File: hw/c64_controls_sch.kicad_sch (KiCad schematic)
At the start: 22 parts, among them J300 DE9_Receptacle, J301 DE9_Receptacle, U300 74AHCT1G125, U301 74AHCT1G125, U302 74AHCT1G125, U303 74AHCT1G125, U304 74AHCT1G125, U305 74AHCT1G125, U306 74AHCT1G125, U307 74AHCT1G125, U308 74AHCT1G125, U309 74AHCT1G125

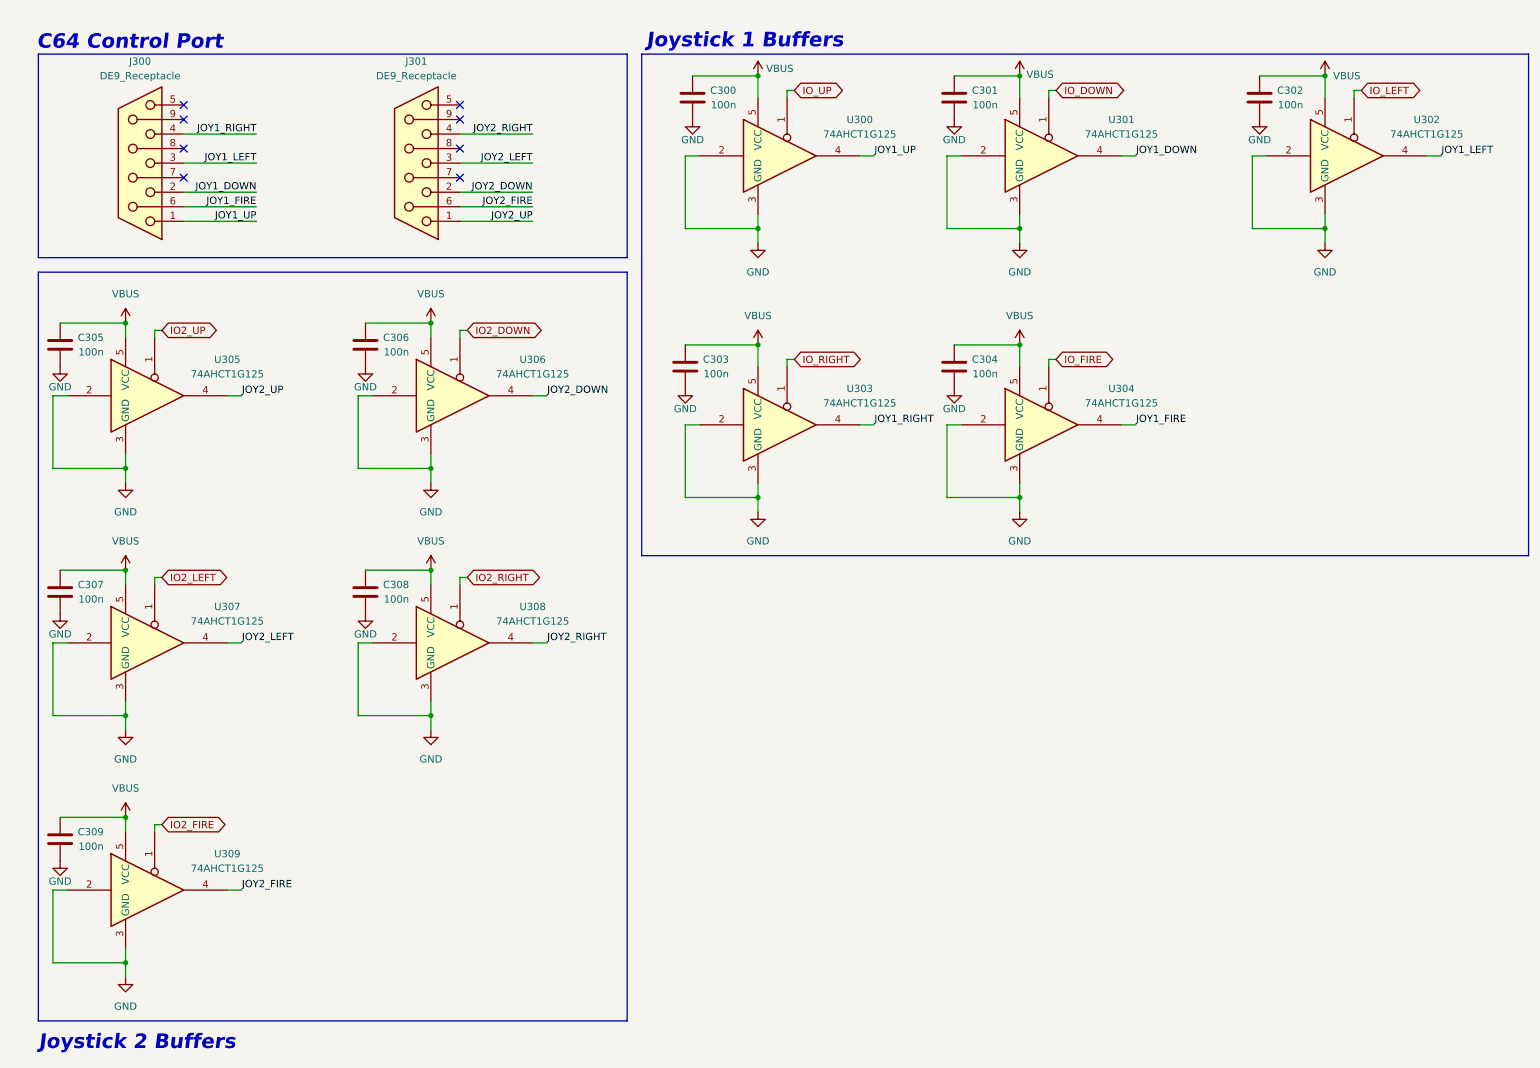
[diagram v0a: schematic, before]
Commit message: 1p version
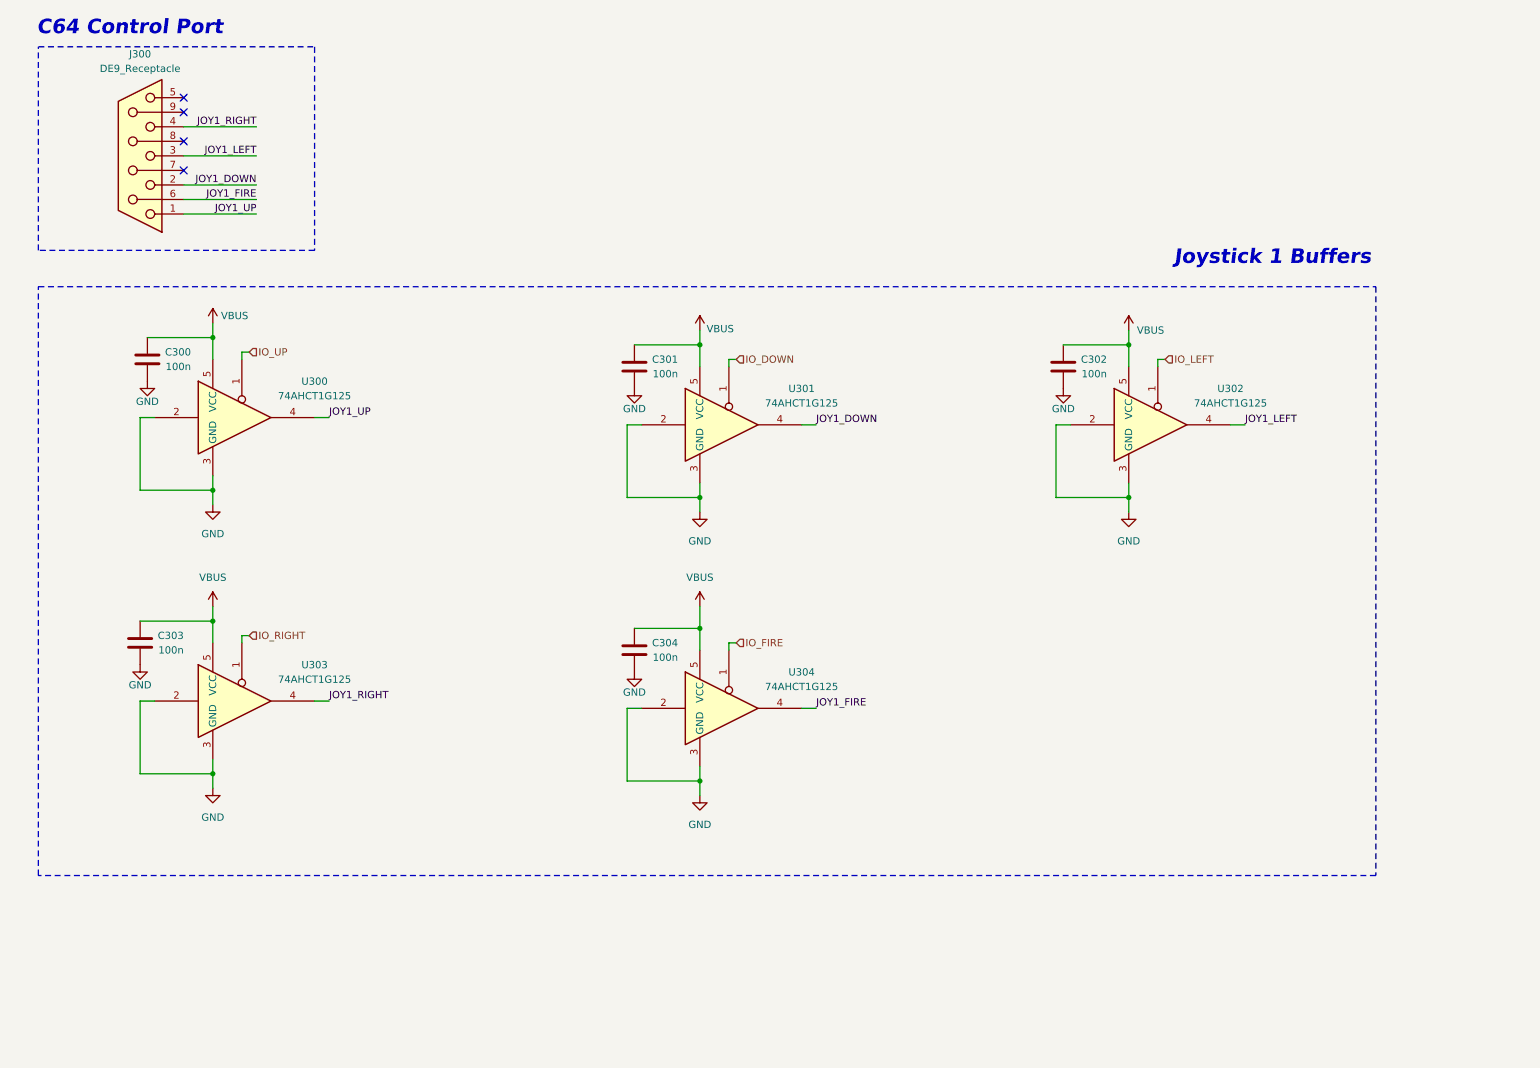
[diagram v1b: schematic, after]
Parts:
- removed C305, C306, C307, C308, C309: 100n, Capacitor_SMD:C_0402_1005Metric, symbol Device:C
- removed J301: DE9_Receptacle, Connector_Dsub:DSUB-9_Female_Horizontal_P2.77x2.84mm_EdgePinOffset4.94mm_Housed_MountingHolesOffset4.94mm, symbol Connector:DE9_Receptacle
- removed U305, U306, U307, U308, U309: 74AHCT1G125, Package_TO_SOT_SMD:SOT-353_SC-70-5, symbol 74xGxx:74AHCT1G125
- J300: footprint Connector_Dsub:DSUB-9_Female_Horizontal_P2.77x2.84mm_EdgePinOffset4.94mm_Housed_MountingHolesOffset4.94mm -> Connector_Dsub:DSUB-9_Female_EdgeMount_P2.77mm
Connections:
- no-connect marks 8 -> 4
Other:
- note removed: "Joystick 2 Buffers"
- moved on the sheet: C300, C301, C302, C303, C304, J300, U300, U301, U302, U303, U304
